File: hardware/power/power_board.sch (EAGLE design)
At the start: 18 parts, among them J1 FASTON_MALE_RA_BLADE, J2 FASTON_MALE_RA_BLADE, J3 12v, J4 5v, J5 XT30PW-F, J6 XT30PW-F, J7 XT30PW-F, J8 XT30PW-F, U1 PDQ30-Q24-S5-D, U2 PDQ30-Q24-S12-D

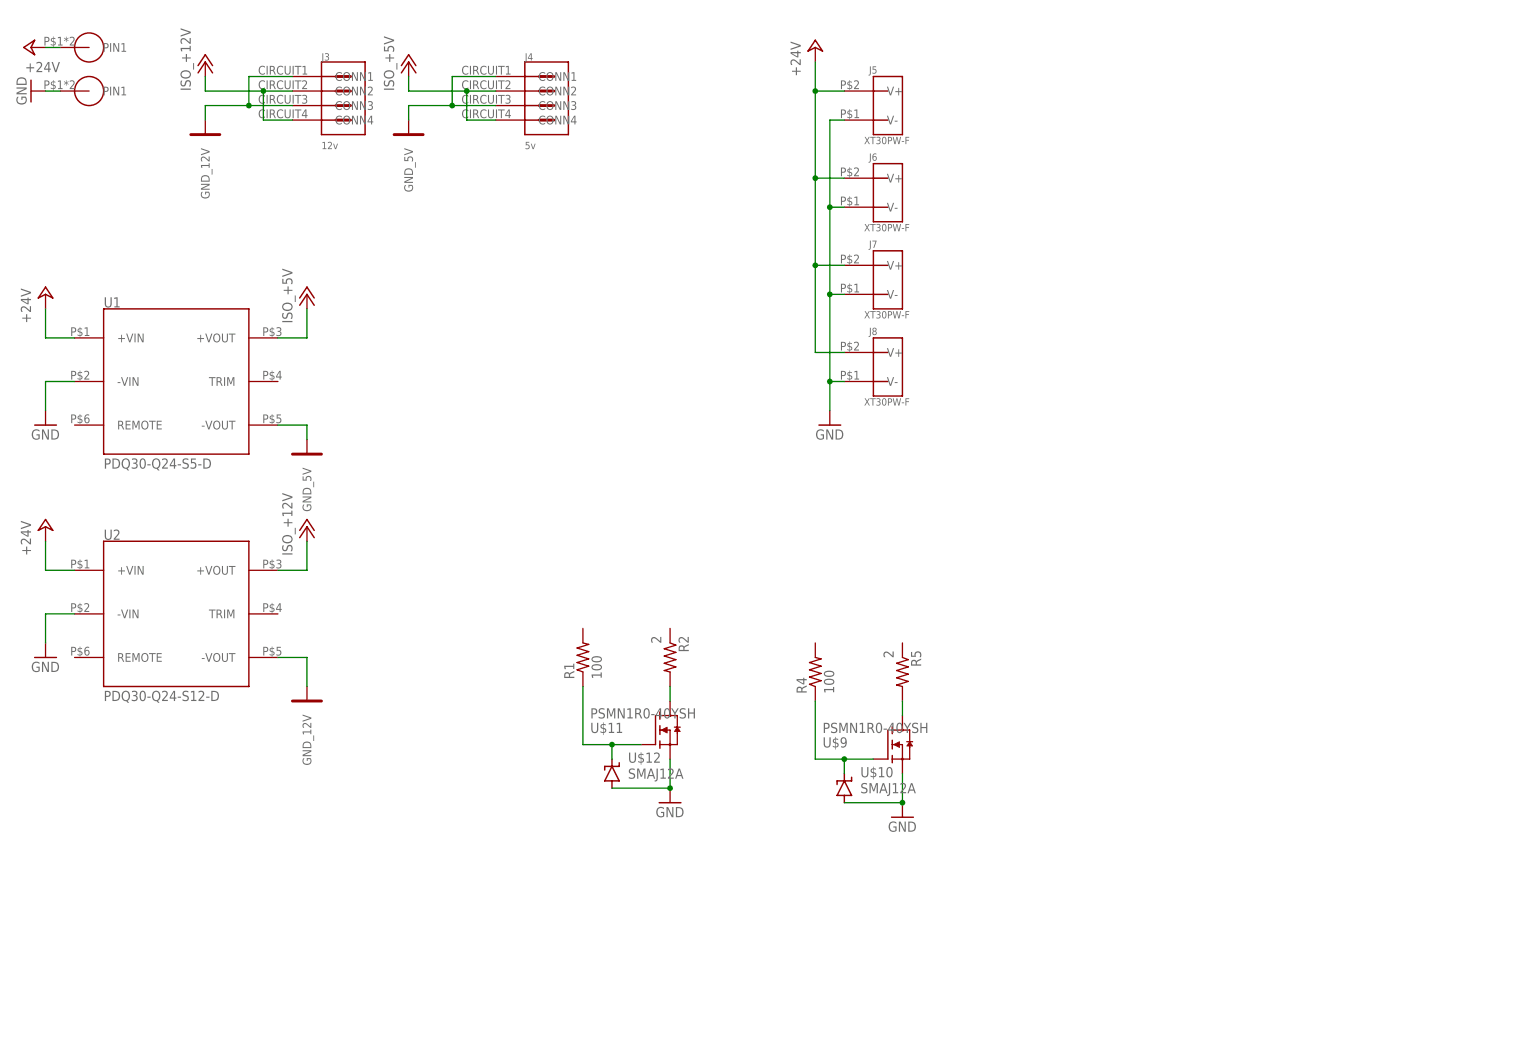
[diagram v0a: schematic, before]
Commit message: Missing some caps
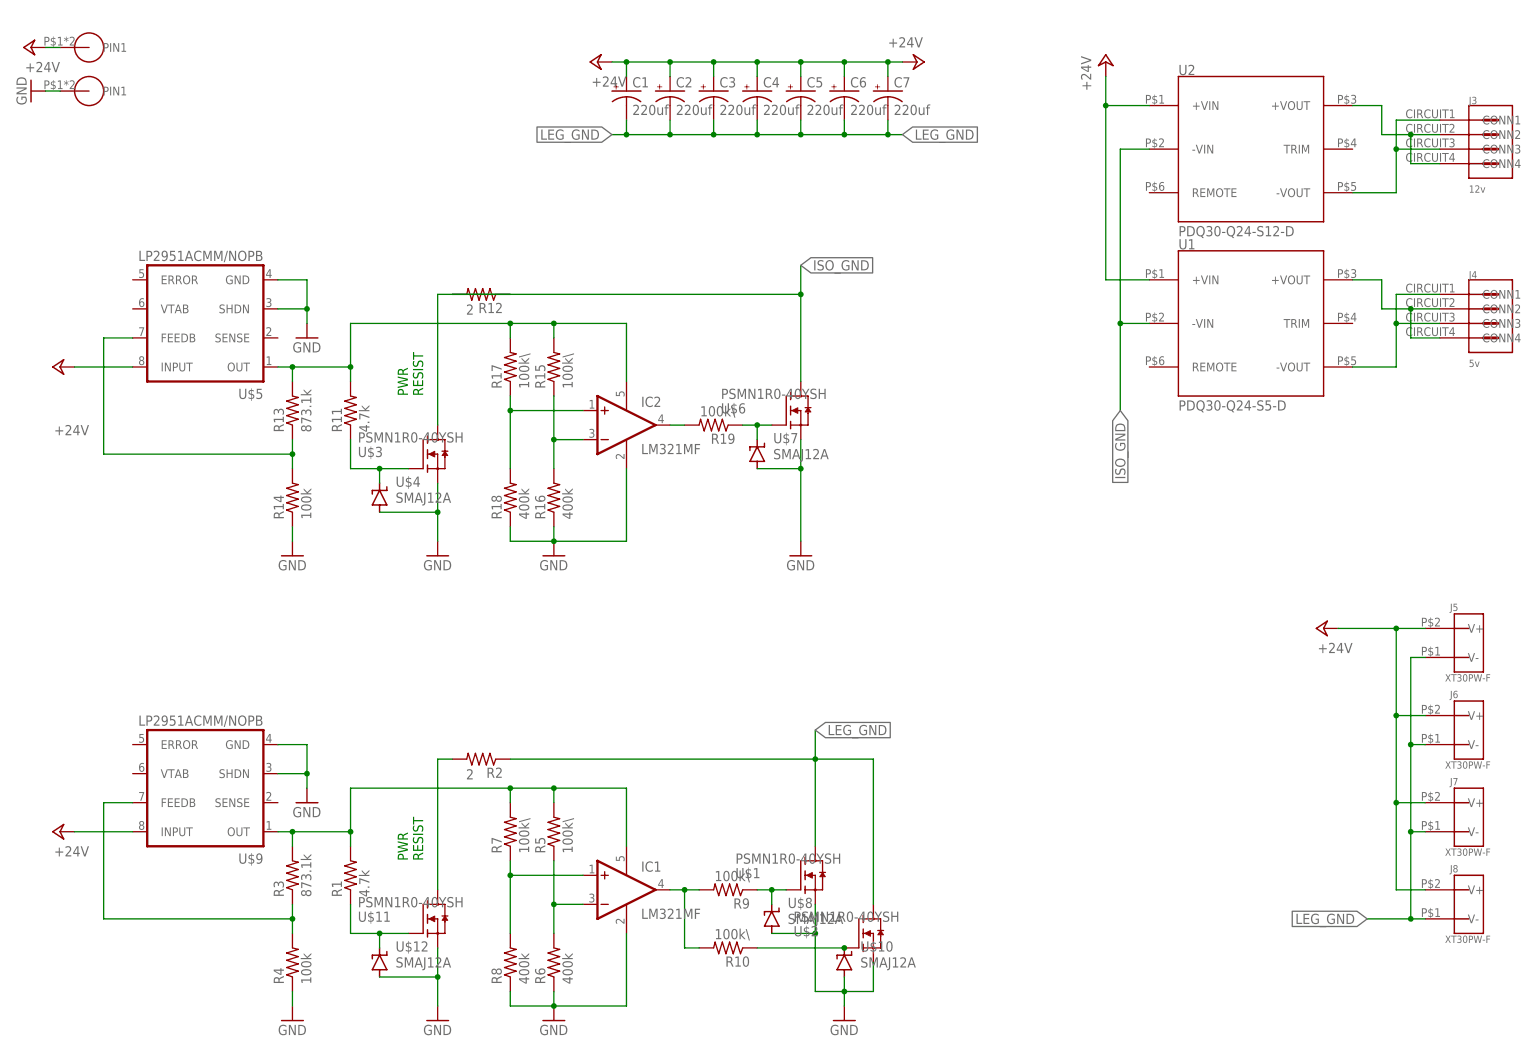
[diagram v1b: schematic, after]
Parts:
- added C1, C2, C3, C4, C5, C6, C7: 220uf, timlib:35ZLH220MEFC8X11.5
- added IC1, IC2: LM321MF, linear:LM321MF
- added R10, R15, R17, R19, R7, R9: 100k\, rcl:R-US_R0603
- added R11: 4.7k, rcl:R-US_R0603
- added R12: 2, timlib:PWR163
- added R13, R3: 873.1k, rcl:R-US_R0603
- added R14: 100k, rcl:R-US_R0603
- added R16, R18, R6, R8: 400k, rcl:R-US_R0603
- added U$1, U$2, U$3, U$6: PSMN1R0-40YSH, timlib:PSMN1R0-40YSH
- added U$4, U$7, U$8: SMAJ12A, timlib:SMAJ12A
- added U$5: LP2951ACMM/NOPB, timlib:LP2951ACMM/NOPB
- R1: value 100 -> 4.7k
- R4: value 100 -> 100k
- R5: value 2 -> 100k\; device timlib:PWR163 -> rcl:R-US_R0603
- U$9: value PSMN1R0-40YSH -> LP2951ACMM/NOPB; device timlib:PSMN1R0-40YSH -> timlib:LP2951ACMM/NOPB
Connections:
- net GND_12V renamed -12VOUT
- net GND_5V renamed -5VOUT
- net ISO_+12V renamed +12VOUT
- net ISO_+5V renamed +5VOUT
- removed net +24V: J1.PIN1, J5.V+, J6.V+, J7.V+, J8.V+, U1.+VIN, U2.+VIN
- new net BATT_+24V: C1.+, C2.+, C3.+, C4.+, C5.+, C6.+, C7.+, J1.PIN1, J5.V+, J6.V+, J7.V+, J8.V+, U$5.INPUT, U$9.INPUT, U1.+VIN, U2.+VIN
- new net BATT_GND: IC1.V-, IC2.V-, J2.PIN1, R14.1, R16.1, R18.1, R4.1, R6.1, R8.1, U$1.S, U$10.A, U$11.S, U$12.A, U$2.S, U$3.S, U$4.A, U$5.GND, U$5.SHDN, U$8.A, U$9.GND, U$9.SHDN
- new net ISO_12V: IC2.V+, R11.2, R13.2, R15.2, R17.2, U$5.OUT
- new net ISO_GND: R12.2, U$6.D, U1.-VIN, U2.-VIN
- new net LEG_12V: IC1.V+, R1.2, R3.2, R5.2, R7.2, U$9.OUT
- new net LEG_GND: C1.-, C2.-, C3.-, C4.-, C5.-, C6.-, C7.-, J5.V-, J6.V-, J7.V-, J8.V-, R2.1, U$1.D, U$2.D
- new net N$10: R13.1, R14.2, U$5.FEEDB
- new net N$11: R12.1, U$3.D
- new net N$12: IC2.-IN, R15.1, R16.2
- new net N$13: IC2.+IN, R17.1, R18.2
- new net N$14: IC2.OUT, R19.2
- new net N$15: R19.1, U$6.G, U$7.C
- new net N$5: IC1.+IN, R7.1, R8.2
- new net N$6: IC1.OUT, R10.2, R9.2
- new net N$7: R11.1, U$3.G, U$4.C
- new net N$8: R9.1, U$1.G, U$8.C
- new net N$9: R10.1, U$10.C, U$2.G
- net GND: now also U$6.S, U$7.A; no longer J2.PIN1, J5.V-, J6.V-, J7.V-, J8.V-, U$10.A, U$11.S, U$12.A, U$9.S, U1.-VIN, U2.-VIN
- net N$3: now also R3.1, R4.2, U$9.FEEDB; no longer R5.2, U$9.D
- net N$4: now also IC1.-IN, R5.1, R6.2; no longer R4.1, U$10.C, U$9.G
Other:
- note added: "PWR RESIST"
- moved on the sheet: J3, J4, J5, J6, J7, J8, R1, R2, R4, R5, U$10, U$11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
